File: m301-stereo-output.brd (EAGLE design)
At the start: 100 x 50 mm, 76 parts, among them U1 SCREW-M2X8, U2 SCREW-M2X8, U3 NUT-M2-SELFLOCK, U4 NUT-M2-SELFLOCK, U5 FX2-20S-1.27DS, U6 ERM1-5MM

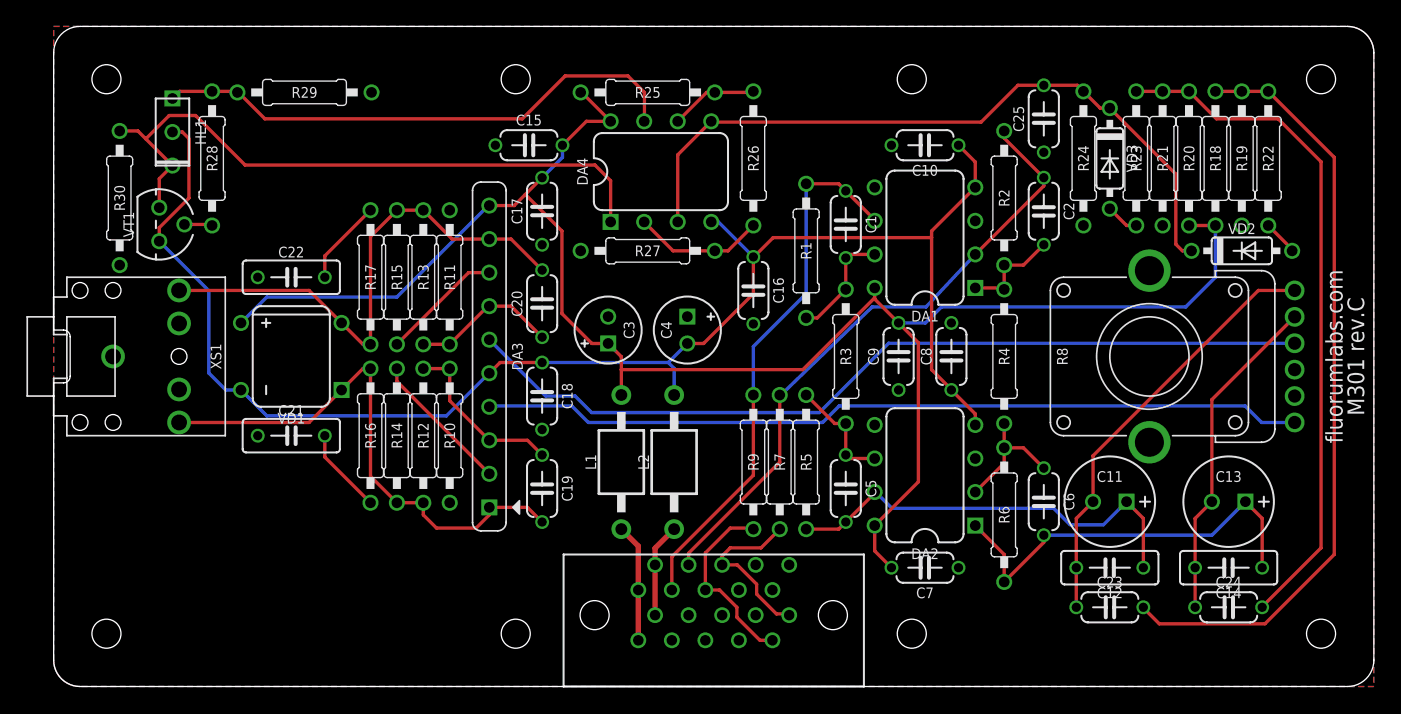
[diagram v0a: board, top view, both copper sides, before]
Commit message: PCB Update
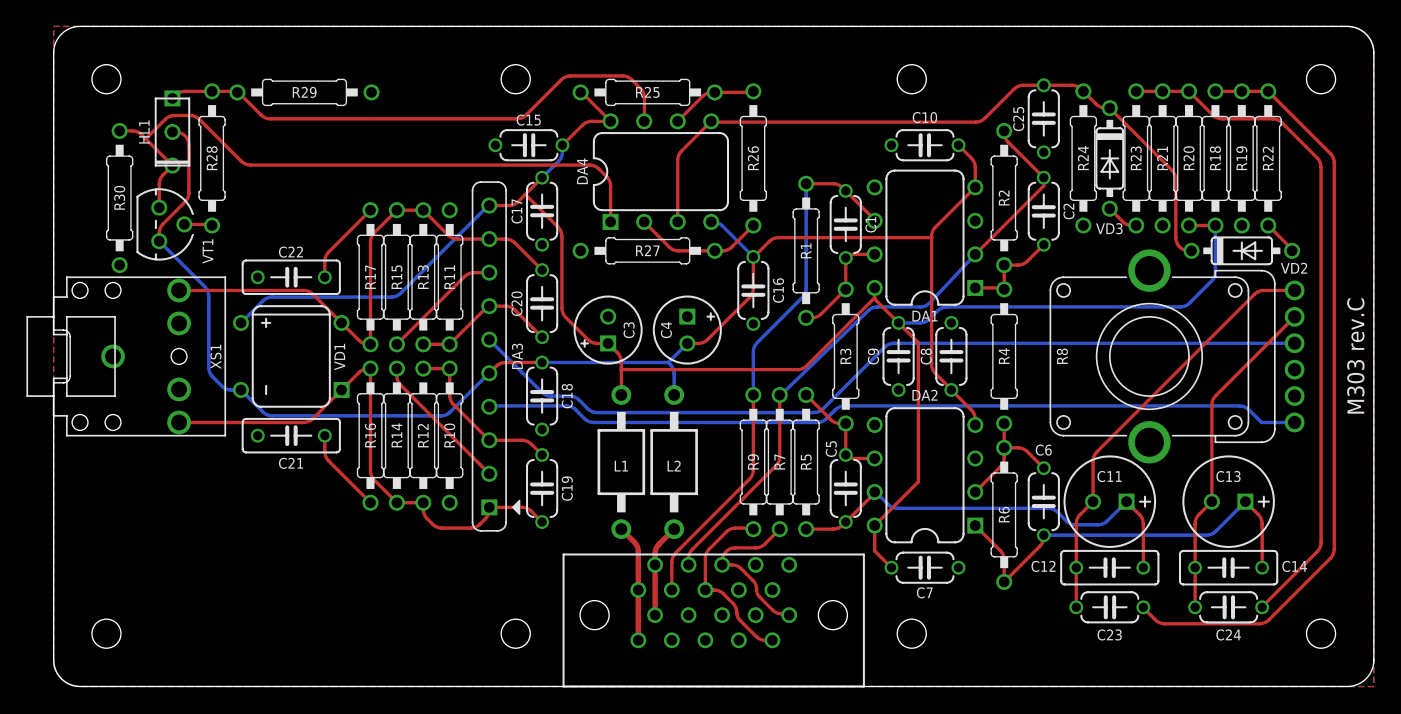
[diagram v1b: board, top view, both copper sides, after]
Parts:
- PCB1: value M301 rev.C -> M303 rev.C
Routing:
- net -15V: track 116.4 -> 115.0 mm
- net +15V: track 134.2 -> 133.3 mm
- net N$21: track 54.5 -> 53.9 mm
- net N$39: track 13.0 -> 12.4 mm
- net N$11: track 41.0 -> 40.5 mm
